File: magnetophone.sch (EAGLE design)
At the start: 22 parts, among them U2 TL072_

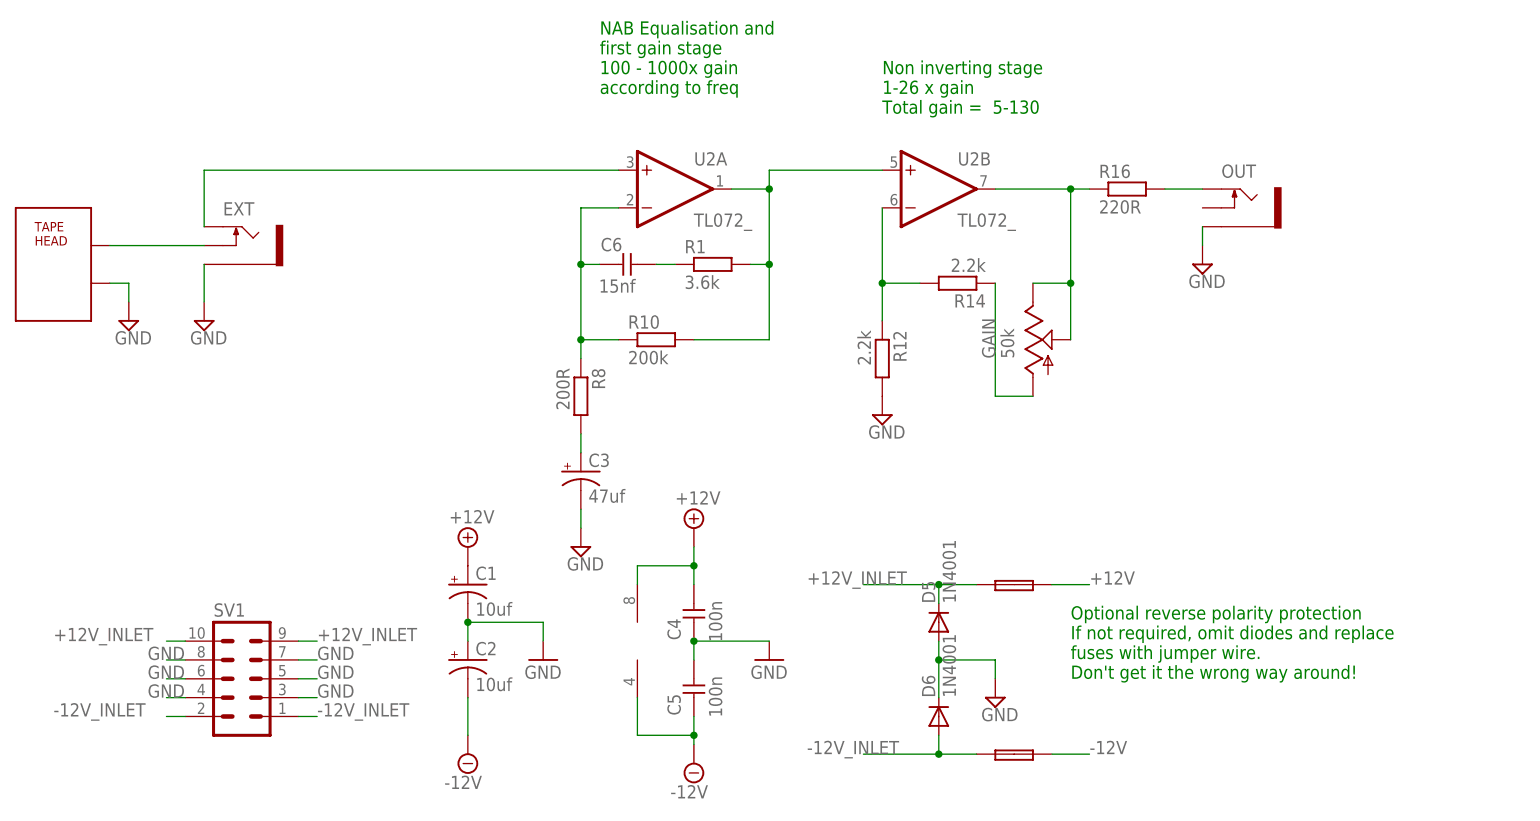
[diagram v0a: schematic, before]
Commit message: First pcb layout
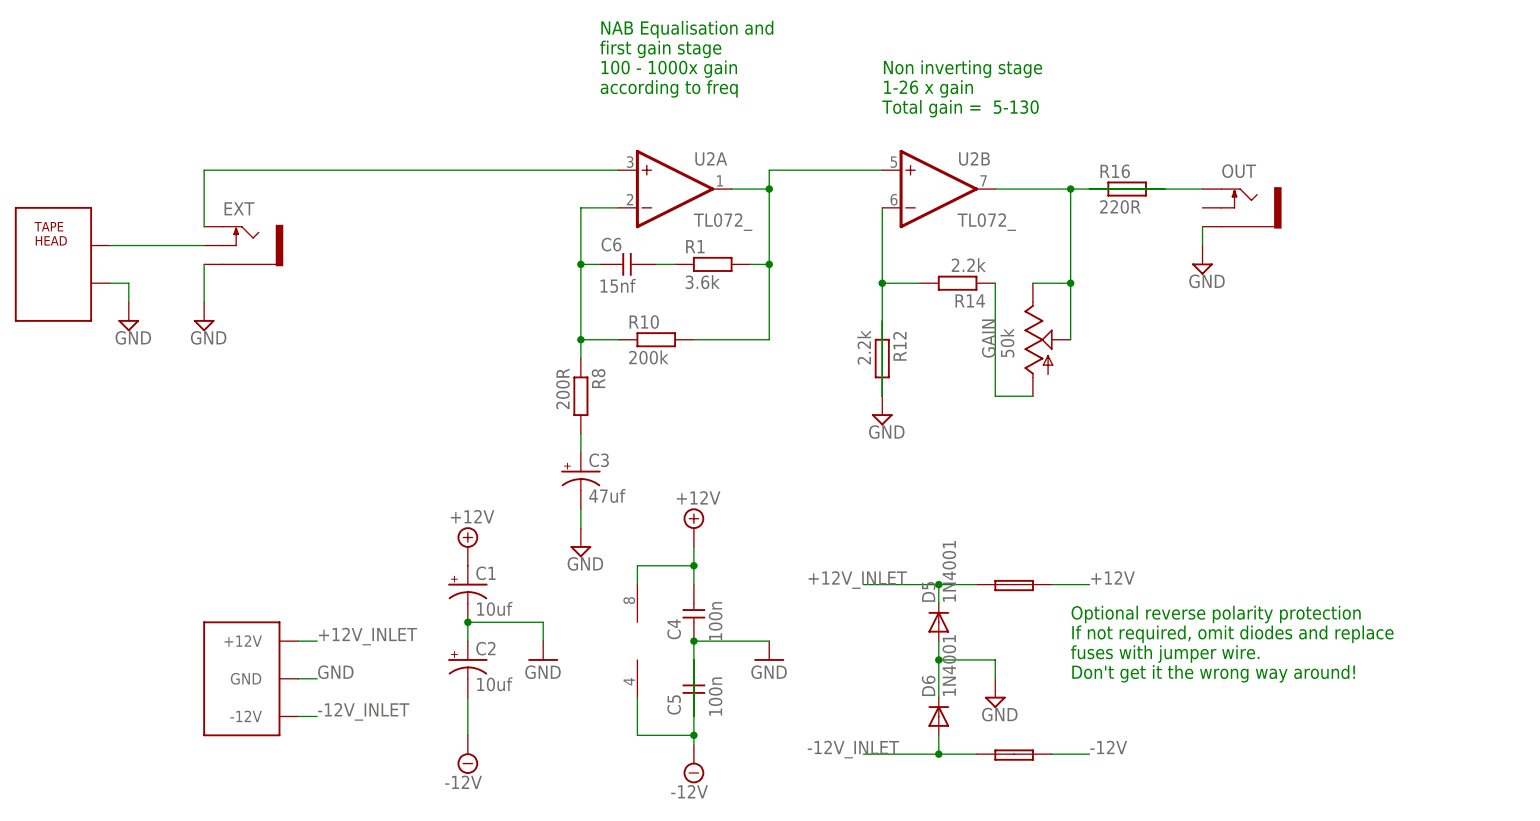
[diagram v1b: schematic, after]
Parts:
- removed SV1: (no value), TomW:10_PIN_HEADER
- added U$2: EURO_POWER_LOCK, MusicThingModular:EURO_POWER_LOCK
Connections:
- net +12V_INLET: now also U$2.+12V; no longer SV1.10, SV1.9
- net -12V: now also C5.1; no longer C5.2
- net -12V_INLET: now also U$2.-12V; no longer SV1.1, SV1.2
- net GND: now also C5.2, R12.1, U$2.GND; no longer C5.1, R12.2, SV1.3, SV1.4, SV1.5, SV1.6, SV1.7, SV1.8
- net N$10: now also R16.1; no longer R16.2
- net N$6: now also R12.2; no longer R12.1
- net N$8: now also R16.2; no longer R16.1
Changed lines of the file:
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@@
 <?xml version="1.0" encoding="utf-8"?>
 <!DOCTYPE eagle SYSTEM "eagle.dtd">
-<eagle version="7.2.0">
+<eagle version="7.4.0">
 <drawing>
 <settings>
@@
 </variantdefs>
 <classes>
-<class number="0" name="default" width="0.6096" drill="0">
+<class number="0" name="default" width="0.3048" drill="0">
 </class>
 <class number="1" name="power" width="0.6096" drill="0">
@@
 <parts>
 <part name="GAIN" library="TomW" deviceset="ALPHA-9MM" device="A" technology="F2" value="50k"/>
-<part name="SV1" library="TomW" deviceset="10_PIN_HEADER" device=""/>
 <part name="SUPPLY3" library="supply2" deviceset="GND" device=""/>
 <part name="R14" library="MusicThingModular" deviceset="RESISTOR" device="7MM" value="2.2k"/>
@@
 <part name="OUT" library="MusicThingModular" deviceset="THONKICONN" device="NEW"/>
 <part name="U2" library="MusicThingModular" deviceset="TL072" device="_"/>
+<part name="U$2" library="MusicThingModular" deviceset="EURO_POWER_LOCK" device=""/>
 </parts>
 <sheets>
@@
 <instance part="U2" gate="B" x="165.1" y="127"/>
 <instance part="GAIN" gate="G$1" x="177.8" y="106.68"/>
-<instance part="SV1" gate="G$1" x="71.12" y="60.96"/>
 <instance part="SUPPLY3" gate="GND" x="66.04" y="109.22"/>
 <instance part="R14" gate="G$1" x="167.64" y="114.3" rot="R180"/>
@@
 <instance part="OUT" gate="G$1" x="205.74" y="124.46"/>
 <instance part="U2" gate="P" x="124.46" y="66.04"/>
+<instance part="U$2" gate="G$1" x="73.66" y="60.96"/>
 </instances>
 <busses>
@@
 <net name="GND" class="2">
 <segment>
-<pinref part="SV1" gate="G$1" pin="7"/>
-<wire x1="81.28" y1="63.5" x2="78.74" y2="63.5" width="0.1524" layer="91"/>
-<label x="81.28" y="63.5" size="1.778" layer="95"/>
-</segment>
-<segment>
-<pinref part="SV1" gate="G$1" pin="5"/>
 <wire x1="81.28" y1="60.96" x2="78.74" y2="60.96" width="0.1524" layer="91"/>
 <label x="81.28" y="60.96" size="1.778" layer="95"/>
-</segment>
-<segment>
-<pinref part="SV1" gate="G$1" pin="3"/>
-<wire x1="81.28" y1="58.42" x2="78.74" y2="58.42" width="0.1524" layer="91"/>
-<label x="81.28" y="58.42" size="1.778" layer="95"/>
-</segment>
-<segment>
-<pinref part="SV1" gate="G$1" pin="8"/>
-<wire x1="60.96" y1="63.5" x2="63.5" y2="63.5" width="0.1524" layer="91"/>
-<label x="58.42" y="63.5" size="1.778" layer="95"/>
-</segment>
-<segment>
-<pinref part="SV1" gate="G$1" pin="6"/>
-<wire x1="60.96" y1="60.96" x2="63.5" y2="60.96" width="0.1524" layer="91"/>
-<label x="58.42" y="60.96" size="1.778" layer="95"/>
-</segment>
-<segment>
-<pinref part="SV1" gate="G$1" pin="4"/>
-<wire x1="60.96" y1="58.42" x2="63.5" y2="58.42" width="0.1524" layer="91"/>
-<label x="58.42" y="58.42" size="1.778" layer="95"/>
+<pinref part="U$2" gate="G$1" pin="GND"/>
 </segment>
 <segment>
@@
 </segment>
 <segment>
-<pinref part="R12" gate="G$1" pin="2"/>
+<pinref part="R12" gate="G$1" pin="1"/>
 <pinref part="SUPPLY5" gate="GND" pin="GND"/>
+<wire x1="157.48" y1="99.06" x2="157.48" y2="109.22" width="0.1524" layer="91"/>
 </segment>
 <segment>
@@
 </segment>
 <segment>
-<wire x1="132.08" y1="63.5" x2="132.08" y2="66.04" width="0.1524" layer="91"/>
+<wire x1="132.08" y1="55.88" x2="132.08" y2="66.04" width="0.1524" layer="91"/>
 <wire x1="132.08" y1="66.04" x2="142.24" y2="66.04" width="0.1524" layer="91"/>
 <pinref part="GND22" gate="1" pin="GND"/>
 <pinref part="C4" gate="G$1" pin="2"/>
 <junction x="132.08" y="66.04"/>
-<pinref part="C5" gate="G$1" pin="1"/>
+<pinref part="C5" gate="G$1" pin="2"/>
 </segment>
 <segment>
@@
 <segment>
 <pinref part="SUPPLY18" gate="G$1" pin="-12V"/>
-<pinref part="C5" gate="G$1" pin="2"/>
+<pinref part="C5" gate="G$1" pin="1"/>
 <wire x1="132.08" y1="52.07" x2="132.08" y2="53.34" width="0.1524" layer="91"/>
-<wire x1="132.08" y1="53.34" x2="132.08" y2="55.88" width="0.1524" layer="91"/>
+<wire x1="132.08" y1="53.34" x2="132.08" y2="63.5" width="0.1524" layer="91"/>
 <wire x1="124.46" y1="58.42" x2="124.46" y2="53.34" width="0.1524" layer="91"/>
 <wire x1="124.46" y1="53.34" x2="132.08" y2="53.34" width="0.1524" layer="91"/>
@@
 <segment>
 <pinref part="U2" gate="B" pin="OUT"/>
-<wire x1="185.42" y1="127" x2="182.88" y2="127" width="0.1524" layer="91"/>
+<wire x1="195.58" y1="127" x2="182.88" y2="127" width="0.1524" layer="91"/>
 <wire x1="182.88" y1="127" x2="172.72" y2="127" width="0.1524" layer="91"/>
-<pinref part="R16" gate="G$1" pin="1"/>
+<pinref part="R16" gate="G$1" pin="2"/>
 <pinref part="GAIN" gate="G$1" pin="S"/>
 <wire x1="182.88" y1="127" x2="182.88" y2="114.3" width="0.1524" layer="91"/>
@@
 <net name="N$10" class="0">
 <segment>
-<pinref part="R16" gate="G$1" pin="2"/>
-<wire x1="200.66" y1="127" x2="195.58" y2="127" width="0.1524" layer="91"/>
+<pinref part="R16" gate="G$1" pin="1"/>
+<wire x1="200.66" y1="127" x2="185.42" y2="127" width="0.1524" layer="91"/>
 <pinref part="OUT" gate="G$1" pin="TIP"/>
 </segment>
@@
 <pinref part="U2" gate="B" pin="-IN"/>
 <wire x1="157.48" y1="124.46" x2="157.48" y2="114.3" width="0.1524" layer="91"/>
-<pinref part="R12" gate="G$1" pin="1"/>
+<pinref part="R12" gate="G$1" pin="2"/>
 <pinref part="R14" gate="G$1" pin="2"/>
-<wire x1="157.48" y1="114.3" x2="157.48" y2="109.22" width="0.1524" layer="91"/>
+<wire x1="157.48" y1="114.3" x2="157.48" y2="99.06" width="0.1524" layer="91"/>
 <wire x1="162.56" y1="114.3" x2="157.48" y2="114.3" width="0.1524" layer="91"/>
 <junction x="157.48" y="114.3"/>
@@
 <net name="+12V_INLET" class="0">
 <segment>
-<pinref part="SV1" gate="G$1" pin="10"/>
-<wire x1="60.96" y1="66.04" x2="63.5" y2="66.04" width="0.1524" layer="91"/>
-<label x="45.72" y="66.04" size="1.778" layer="95"/>
-</segment>
-<segment>
-<pinref part="SV1" gate="G$1" pin="9"/>
 <wire x1="81.28" y1="66.04" x2="78.74" y2="66.04" width="0.1524" layer="91"/>
 <label x="81.28" y="66.04" size="1.778" layer="95"/>
+<pinref part="U$2" gate="G$1" pin="+12V"/>
 </segment>
 <segment>
@@
 <net name="-12V_INLET" class="0">
 <segment>
-<pinref part="SV1" gate="G$1" pin="1"/>
 <wire x1="81.28" y1="55.88" x2="78.74" y2="55.88" width="0.1524" layer="91"/>
 <label x="81.28" y="55.88" size="1.778" layer="95"/>
-</segment>
-<segment>
-<pinref part="SV1" gate="G$1" pin="2"/>
-<wire x1="60.96" y1="55.88" x2="63.5" y2="55.88" width="0.1524" layer="91"/>
-<label x="45.72" y="55.88" size="1.778" layer="95"/>
-</segment>
-<segment>
+<pinref part="U$2" gate="G$1" pin="-12V"/>
+</segment>
+<segment>
